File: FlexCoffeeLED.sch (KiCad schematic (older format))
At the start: 32 parts, among them IC1 NCP718ASN330T1G, IC2 PIC18F25K80-I_SO, IC3 MCP9904T-AE_9Q, J1 Conn_01x05_Male, J2 Conn_01x01_Male, J3 Conn_01x01_Male, Q1 2N3904, Q2 2N3904, Q3 2N3904, U1 PCA9306

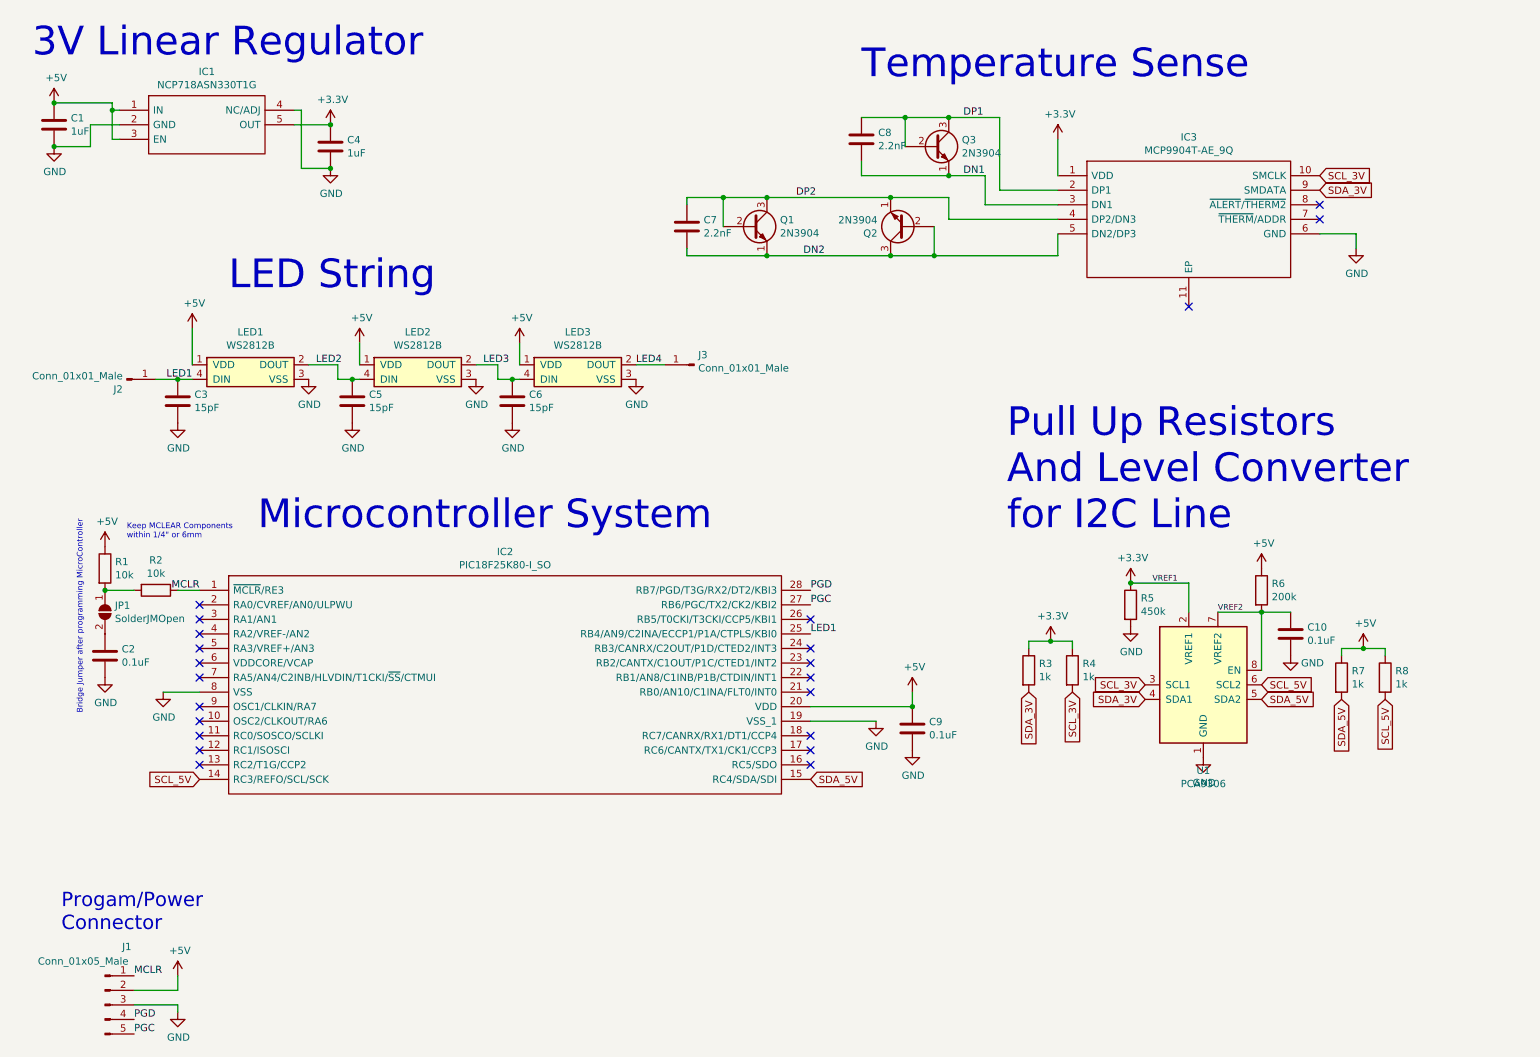
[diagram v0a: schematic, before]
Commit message: A Brand New Design
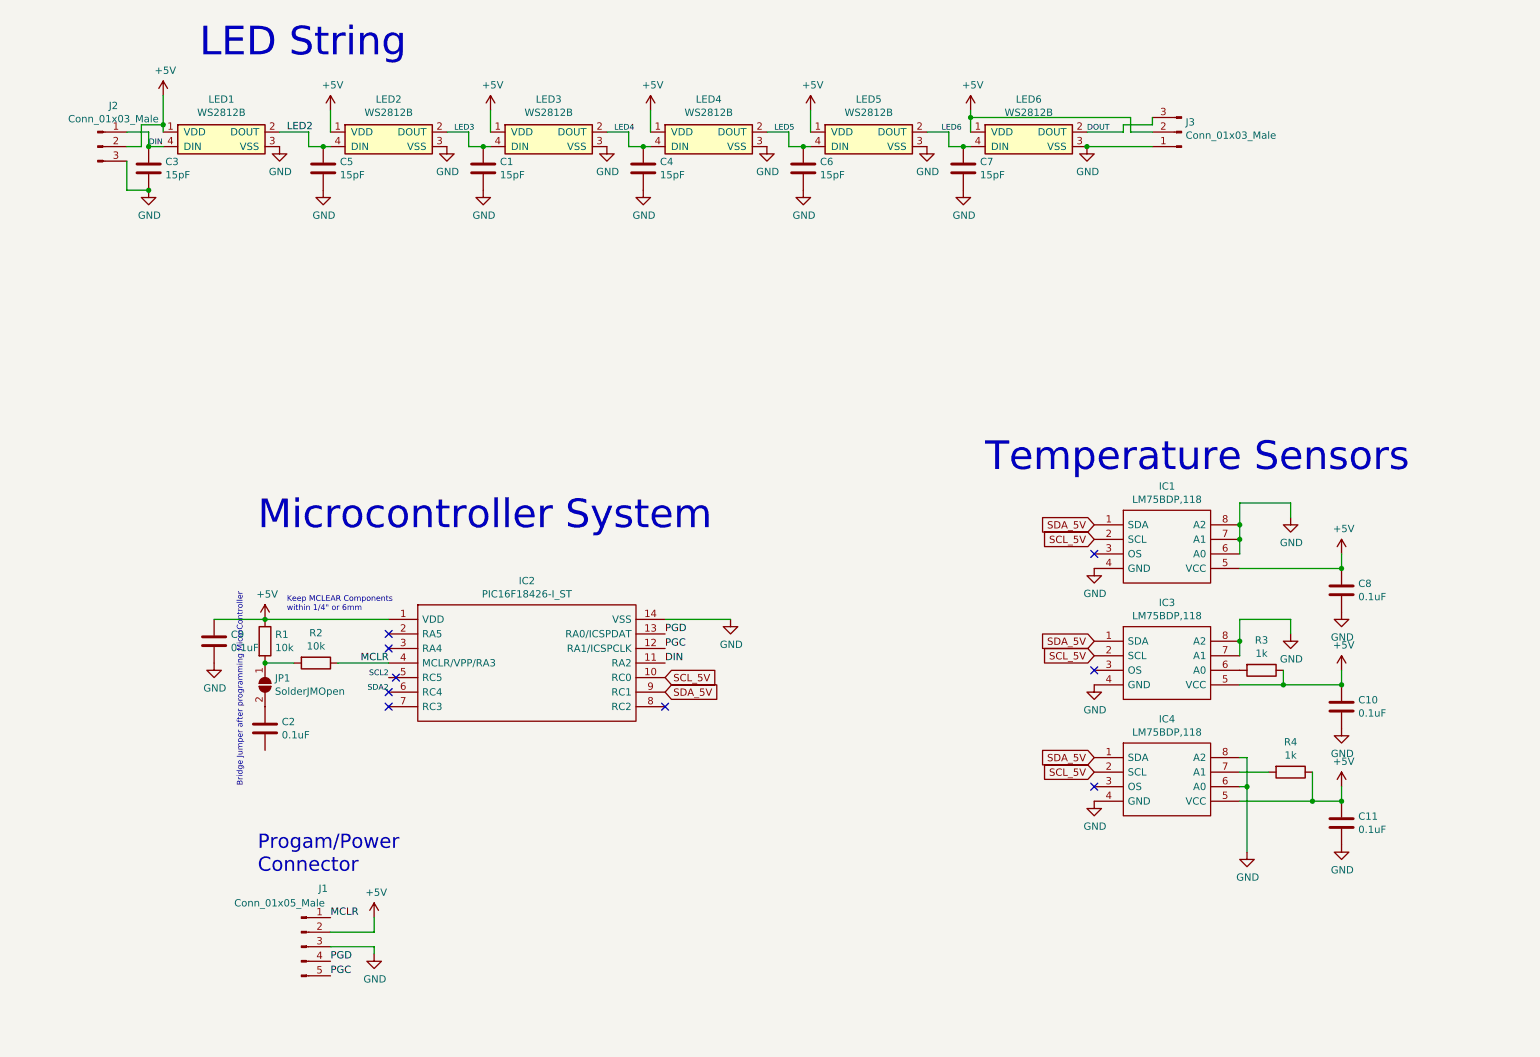
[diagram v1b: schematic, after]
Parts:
- removed IC1: NCP718ASN330T1G, SamacSys_Parts:SOT95P280X100-5N, symbol SamacSys_Parts:NCP718ASN330T1G
- removed IC2: PIC18F25K80-I_SO, SamacSys_Parts:SOIC127P1030X265-28N, symbol SamacSys_Parts:PIC18F25K80-I_SO
- removed IC3: MCP9904T-AE_9Q, SamacSys_Parts:SON50P300X300X90-11N-D, symbol SamacSys_Parts:MCP9904T-AE_9Q
- removed J2, J3: Conn_01x01_Male, Pin_Headers:Pin_Header_Straight_1x01_Pitch2.54mm, symbol Connector:Conn_01x01_Male
- removed Q1, Q2, Q3: 2N3904, TO_SOT_Packages_THT:TO-92_Inline_Narrow_Oval, symbol Transistor_BJT:2N3904
- removed R5: 450k, Resistors_SMD:R_0603, symbol device:R
- removed R6: 200k, Resistors_SMD:R_0603, symbol device:R
- removed R7, R8: 1k, Resistors_SMD:R_0603, symbol device:R
- removed U1: PCA9306, SamacSys_Parts:SOP50P310X90-8N, symbol interface:PCA9306
- added C11: 0.1uF, Capacitors_SMD:C_0603, symbol device:C
- added IC1, IC3, IC4: LM75BDP,118, SamacSys_Parts:SOP65P490X110-8N, symbol SamacSys_Parts:LM75BDP,118
- added IC2: PIC16F18426-I_ST, SOP65P640X120-14N, symbol SamacSys_Parts:PIC16F18426-I_ST
- added J2, J3: Conn_01x03_Male, Pin_Headers:Pin_Header_Straight_1x03_Pitch2.54mm, symbol Connector:Conn_01x03_Male
- added LED4, LED5, LED6: WS2812B, LEDs:LED_WS2812B-PLCC4, symbol Worldsemi:WS2812B
- C1, C4: value 1uF -> 15pF
- C7: value 2.2nF -> 15pF
- C8: value 2.2nF -> 0.1uF
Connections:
- net DN1 is gone; now on net GND: C8.2
- net DN2 is gone; now on net GND: C7.2
- net DP1 is gone; now on net +5V: C8.1
- net VREF2 is gone; now on net +5V: C10.1
- net +5V: now also R3.1, R4.1, C11.1, IC1.5 (VCC), IC2.1 (VDD), IC3.5 (VCC), IC4.5 (VCC), J2.2 (Pin_2), J3.2 (Pin_2), LED4.1 (VDD), LED5.1 (VDD), LED6.1 (VDD); no longer C1.1
- net GND: now also C11.2, IC1.4 (GND), IC1.6 (A0), IC1.7 (A1), IC1.8 (A2), IC2.14 (VSS), IC3.4 (GND), IC3.7 (A1), IC3.8 (A2), IC4.4 (GND), IC4.6 (A0), IC4.8 (A2), J2.3 (Pin_3), J3.1 (Pin_1), LED4.3 (VSS), LED5.3 (VSS), LED6.3 (VSS); no longer C2.2
- net LED3: now also C1.1; no longer C6.1
- net LED4: now also C4.1, LED4.4 (DIN)
- net MCLR: now also IC2.4 (MCLR/VPP/RA3)
- net PGC: now also IC2.12 (RA1/ICSPCLK)
- net PGD: now also IC2.13 (RA0/ICSPDAT)
- net SCL_5V: now also IC1.2 (SCL), IC2.10 (RC0), IC3.2 (SCL), IC4.2 (SCL)
- net SDA_5V: now also IC1.1 (SDA), IC2.9 (RC1), IC3.1 (SDA), IC4.1 (SDA)
- removed net +3V3: C4.1, R3.1, R4.1
- net DP2 renamed LED6
- net LED6: now also LED5.2 (DOUT), LED6.4 (DIN)
- net LED1 renamed DIN
- net DIN: now also IC2.11 (RA2), J2.1 (Pin_1)
- net SCL_3V: no longer names the net of R4.2
- net SCL_3V: now also IC4.7 (A1)
- net SDA_3V: no longer names the net of R3.2
- net SDA_3V: now also IC3.6 (A0)
- new net DOUT: J3.3 (Pin_3), LED6.2 (DOUT)
- new net LED5: C6.1, LED4.2 (DOUT), LED5.4 (DIN)
- new net SCL2: IC2.5 (RC5)
- new net SDA2: IC2.6 (RC4)
- no-connect marks 22 -> 9
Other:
- note added: "Temperature Sensors"
- note removed: "3V Linear Regulator"
- note removed: "Pull Up Resistors \nAnd Level Converter\nfor I2C Line"
- note removed: "Temperature Sense"
- moved on the sheet: C2, C3, C5, C9, J1, JP1, LED1, LED2, R1, R2
